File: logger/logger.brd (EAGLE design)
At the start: 100 x 80 mm, 27 parts, among them IC1 75176AD, IC2 REG1117, U1 MSP430G2352IPW14

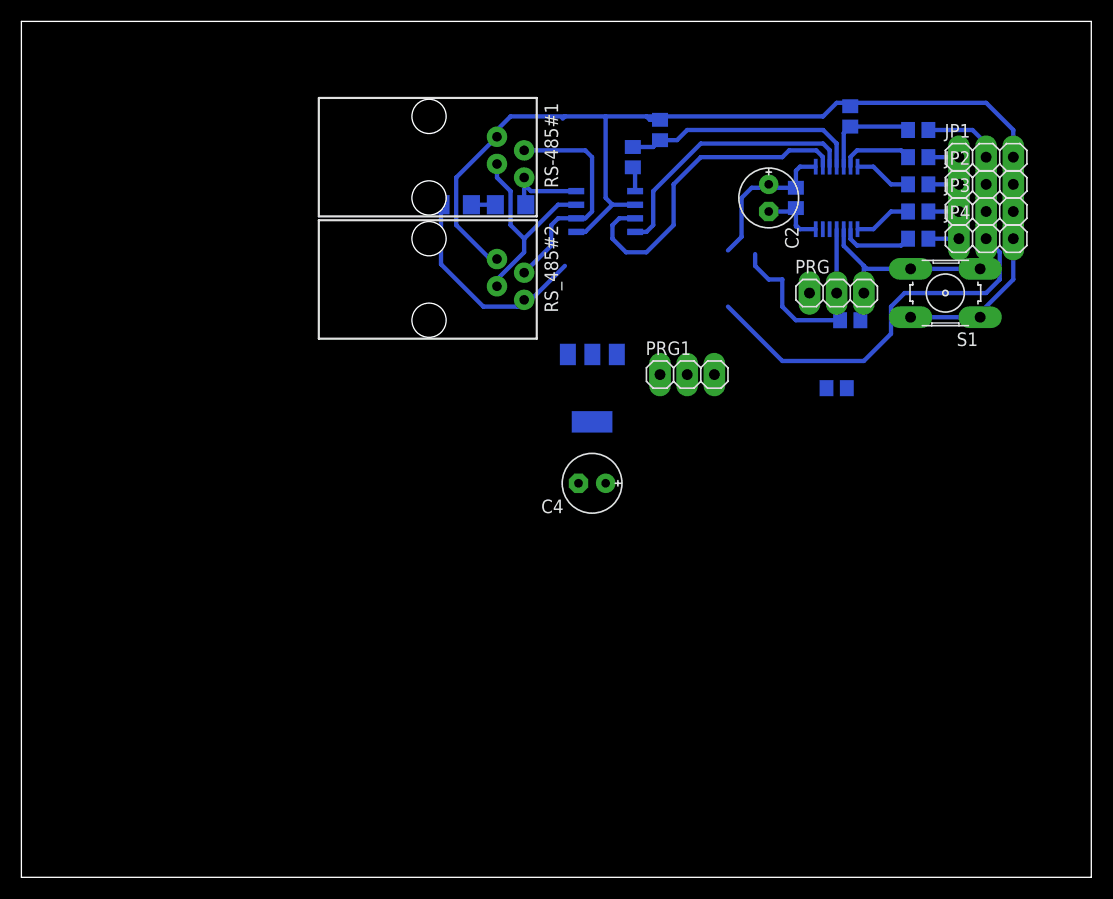
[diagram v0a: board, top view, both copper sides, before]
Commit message: Routed.
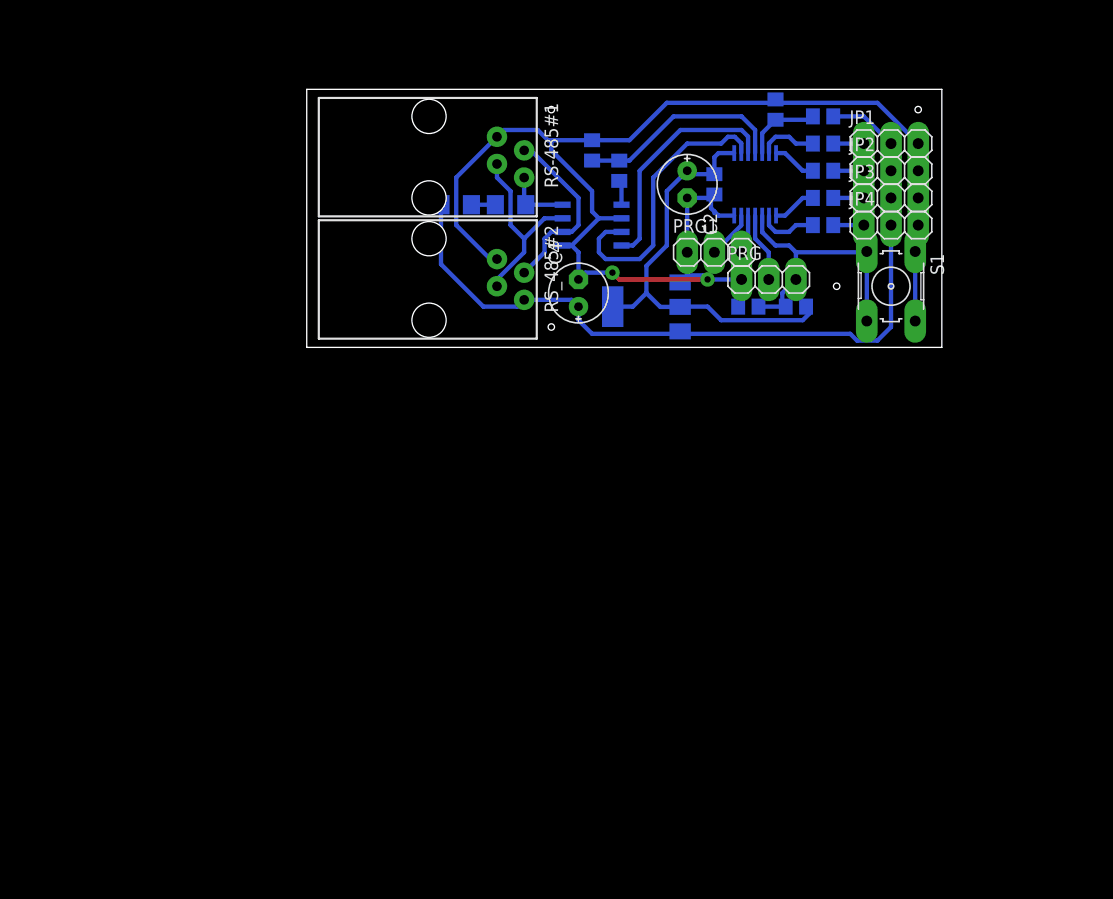
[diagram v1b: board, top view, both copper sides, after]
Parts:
- moved C4 17.8 mm to (52.1, 54.6), turned to 90 degrees
- moved PRG1 11.7 mm to (64.8, 58.4)
- moved C3 11.2 mm to (67.9, 53.3)
- moved IC2 9.16 mm to (58.4, 53.3), turned to 270 degrees
- moved JP2 8.98 mm to (81.3, 66.0)
- moved JP3 8.98 mm to (81.3, 63.5)
- moved JP4 8.98 mm to (81.3, 61.0)
- moved JP1 8.98 mm to (81.3, 68.6)
- moved R2 8.98 mm to (74.9, 66.0)
- moved R5 8.98 mm to (74.9, 71.1)
- moved R1 8.98 mm to (74.9, 68.6)
- moved R3 8.98 mm to (74.9, 63.5)
- moved R4 8.98 mm to (74.9, 61.0)
- moved C1 7.73 mm to (64.8, 64.8)
- moved U1 7.73 mm to (68.6, 64.8)
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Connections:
- removed net N$17: PRG1.1, U1.13
- new net N$12: PRG1.2, U1.13
- net +3V3: now also IC2.4
- net GND: now also PRG1.1; no longer PRG1.3
- net N$18: now also PRG1.3; no longer PRG1.2
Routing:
- net GND: track 114.9 -> 129.0 mm, vias 0 -> 2
- net +3V3: track 27.6 -> 40.3 mm
- net N$15: track 20.4 -> 26.9 mm
- net +5V: track 79.3 -> 83.8 mm
- net N$12: track 0.00 -> 4.47 mm
- net N$1: track 21.5 -> 17.1 mm
- net N$14: track 31.2 -> 26.8 mm
- net N$18: track 0.00 -> 3.68 mm
- net N$13: track 25.3 -> 21.8 mm
- net N$22: track 22.4 -> 19.6 mm
- net N$3: track 9.53 -> 7.26 mm
- net N$2: track 19.7 -> 17.9 mm
- net N$20: track 7.74 -> 6.05 mm
- net N$10: track 5.40 -> 4.13 mm
- net N$4: track 6.80 -> 5.53 mm
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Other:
- board size 100 x 80 mm -> 59.4 x 24.1 mm
